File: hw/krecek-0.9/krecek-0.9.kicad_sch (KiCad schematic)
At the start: 3 parts, among them J1 USB_C_Receptacle_USB2.0, U1 RP2040, U2 W25Q128JVS

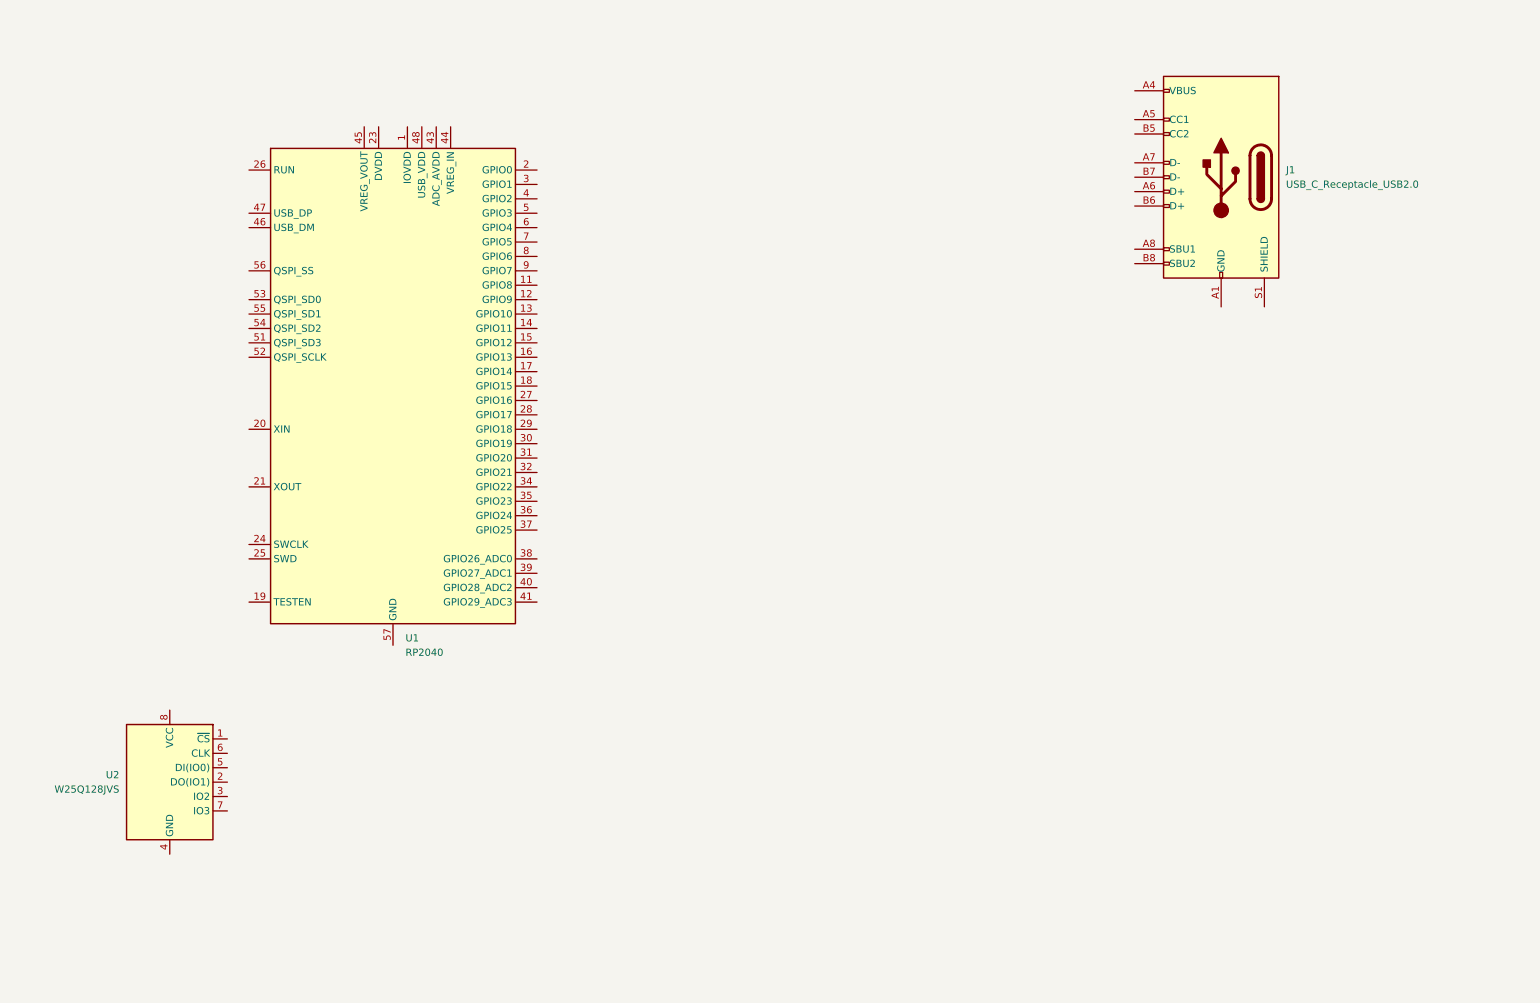
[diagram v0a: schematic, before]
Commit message: Expert hardware design *dab*
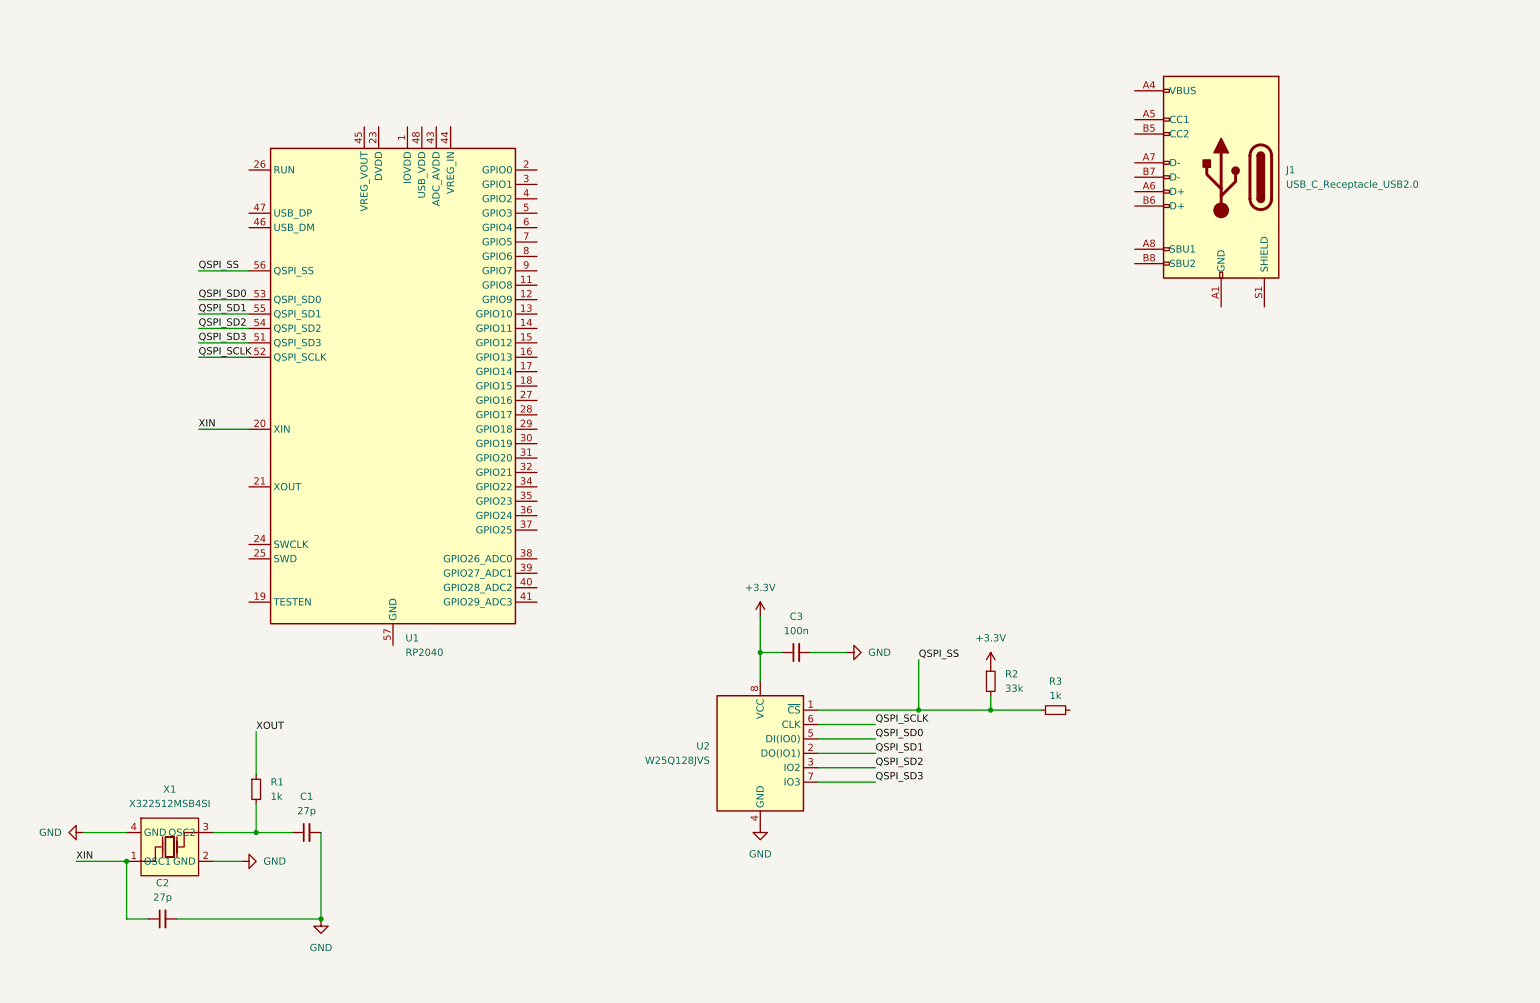
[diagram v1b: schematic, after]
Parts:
- added C1, C2: 27p, symbol Device:C_Small
- added C3: 100n, symbol Device:C_Small
- added R1, R3: 1k, symbol Device:R_Small
- added R2: 33k, symbol Device:R_Small
- added X1: X322512MSB4SI, LCSC:OSC-SMD_4P-L3.2-W2.5-BL, symbol LCSC:X322512MSB4SI
- J1: footprint (none) -> LCSC:USB-C-SMD_TYPEC-304J-BCP16; LCSC Part (none) -> C2835315
- U1: LCSC Part (none) -> C2040
- U2: LCSC Part (none) -> C97521
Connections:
- net XIN: now reaches U1.20 (XIN)
- net XIN: now also C2.1, X1.1 (OSC1)
- net QSPI_SD3: now reaches U1.51 (QSPI_SD3)
- net QSPI_SD3: now also U2.7 (IO3)
- net QSPI_SCLK: now reaches U1.52 (QSPI_SCLK)
- net QSPI_SCLK: now also U2.6 (CLK)
- net QSPI_SD0: now reaches U1.53 (QSPI_SD0)
- net QSPI_SD0: now also U2.5 (DI(IO0))
- net QSPI_SD2: now reaches U1.54 (QSPI_SD2)
- net QSPI_SD2: now also U2.3 (IO2)
- net QSPI_SD1: now reaches U1.55 (QSPI_SD1)
- net QSPI_SD1: now also U2.2 (DO(IO1))
- net QSPI_SS: now reaches U1.56 (QSPI_SS)
- net QSPI_SS: now also U2.1 (~{CS}), R2.2, R3.1
- net GND: now reaches U2.4 (GND)
- net GND: now also C1.2, C2.2, C3.2, X1.2 (GND), X1.4 (GND)
- net +3.3V: now reaches U2.8 (VCC)
- net +3.3V: now also C3.1, R2.1
- new net: C1.1, R1.2, X1.3 (OSC2)
- new net XOUT: R1.1
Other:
- moved on the sheet: U2

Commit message: expand design
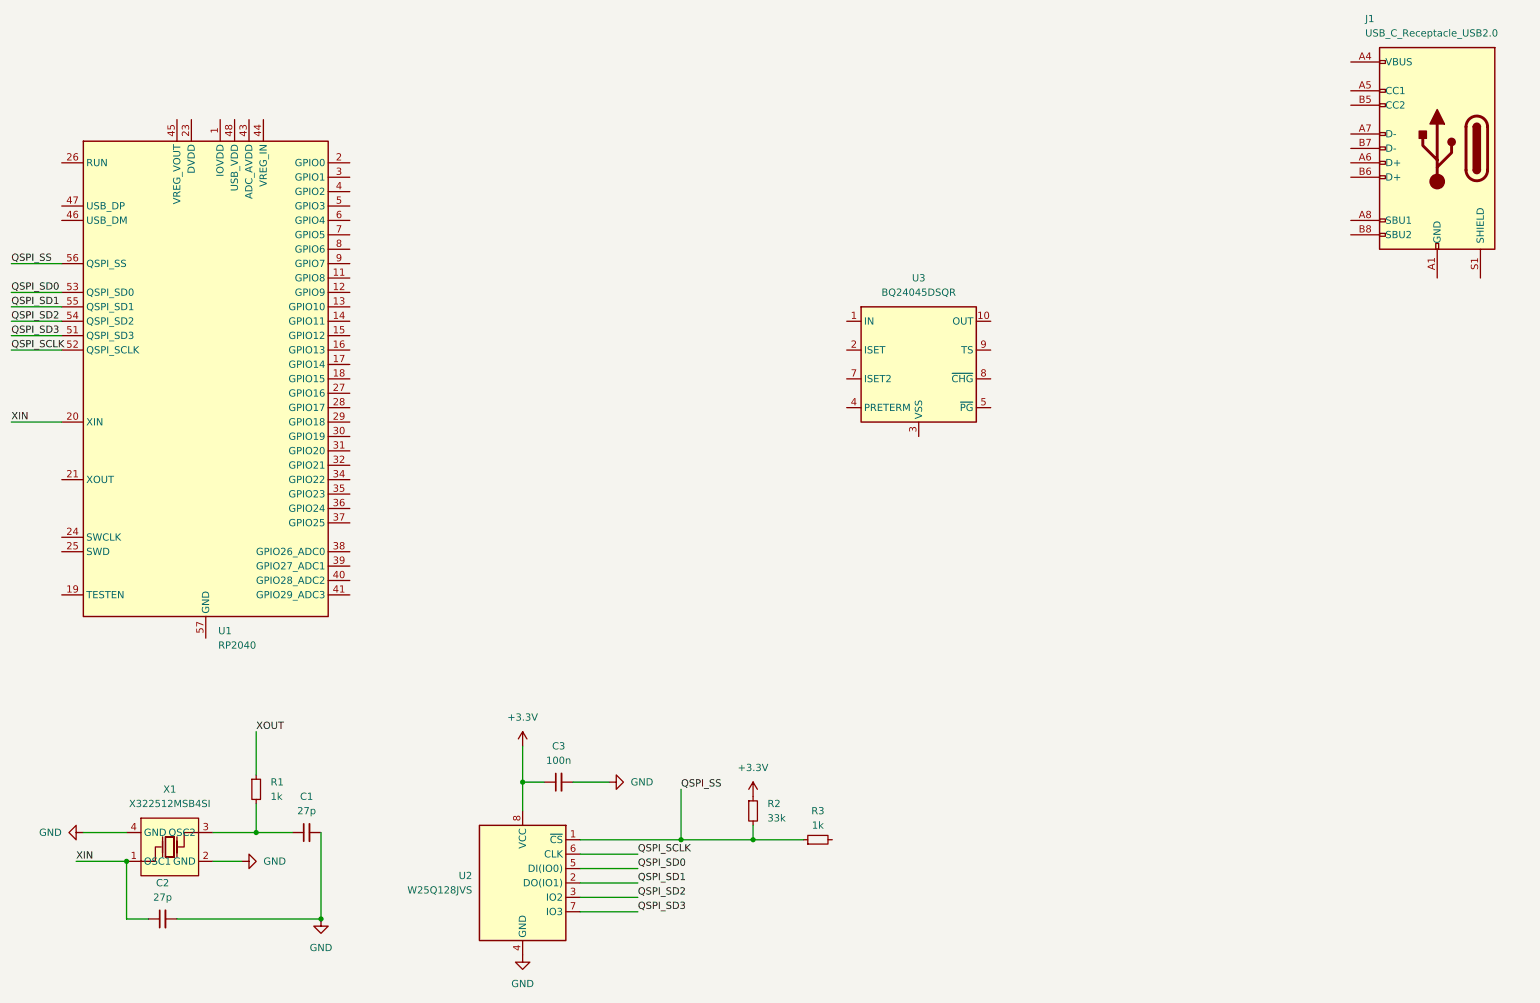
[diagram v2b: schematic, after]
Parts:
- added U3: BQ24045DSQR, LCSC:WSON-10_L2.0-W2.0-P0.40-BL-EP, symbol LCSC:BQ24045DSQR
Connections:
- new net: U3.11 (VSS), U3.3 (VSS)
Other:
- moved on the sheet: C3, J1, R2, R3, U1, U2

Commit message: assign GPIO pins
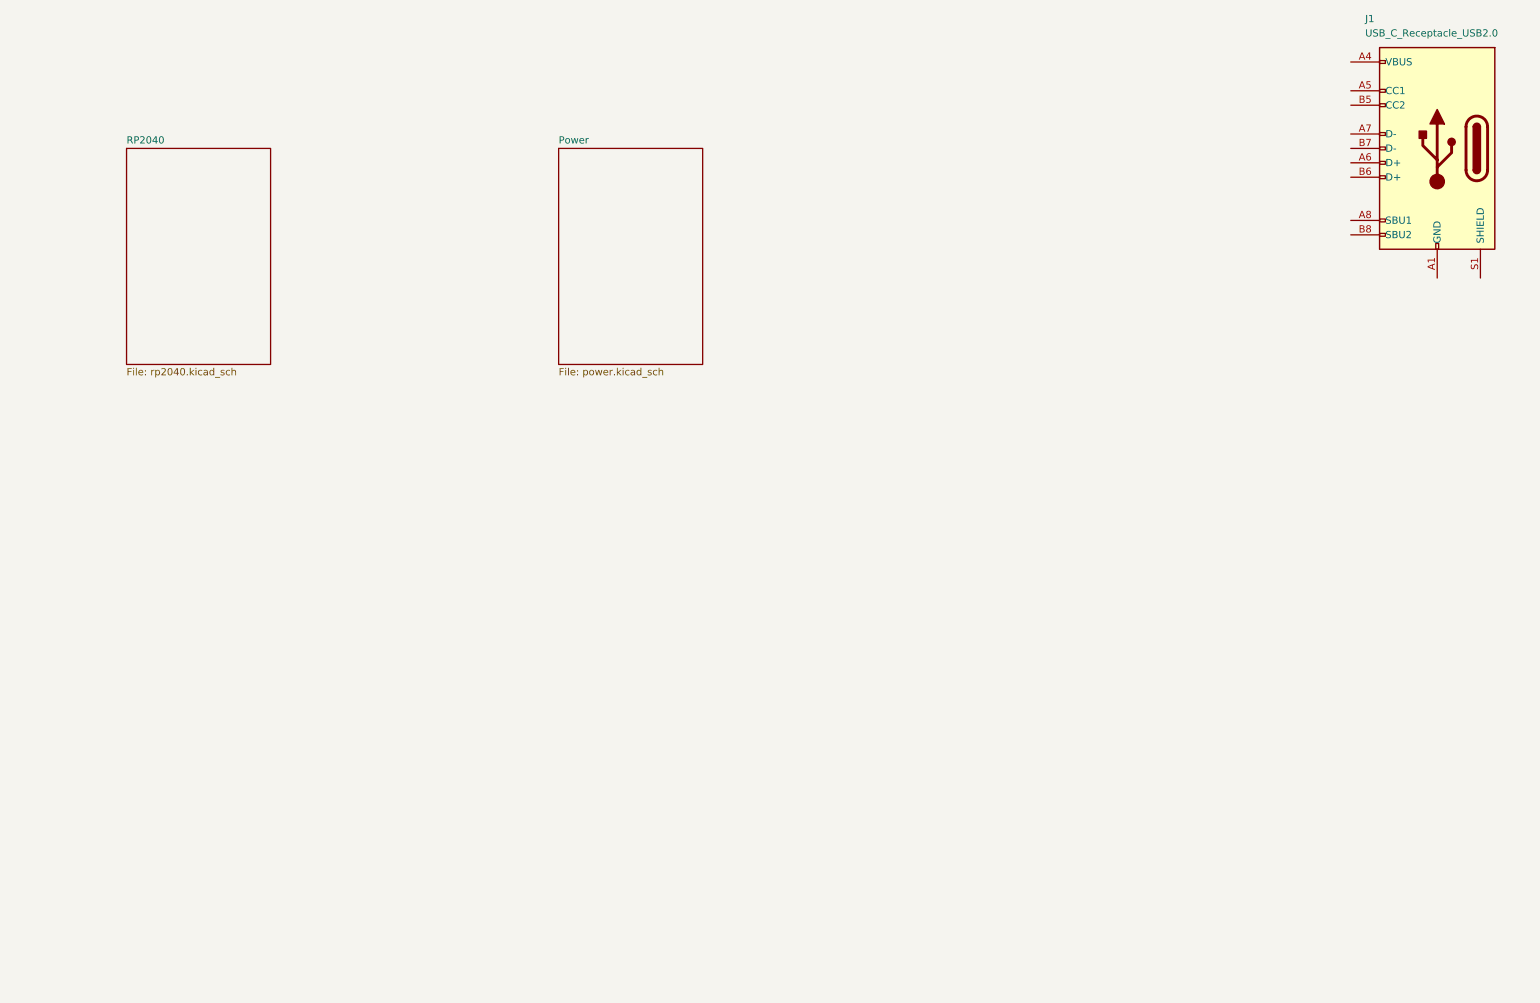
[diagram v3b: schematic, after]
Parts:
- removed C1, C2: 27p, symbol Device:C_Small
- removed C3: 100n, symbol Device:C_Small
- removed R1, R3: 1k, symbol Device:R_Small
- removed R2: 33k, symbol Device:R_Small
- removed U1: RP2040, Package_DFN_QFN:QFN-56-1EP_7x7mm_P0.4mm_EP3.2x3.2mm, symbol MCU_RaspberryPi:RP2040
- removed U2: W25Q128JVS, Package_SO:SOIC-8_5.23x5.23mm_P1.27mm, symbol Memory_Flash:W25Q128JVS
- removed U3: BQ24045DSQR, LCSC:WSON-10_L2.0-W2.0-P0.40-BL-EP, symbol LCSC:BQ24045DSQR
- removed X1: X322512MSB4SI, LCSC:OSC-SMD_4P-L3.2-W2.5-BL, symbol LCSC:X322512MSB4SI
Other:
- added sheet Power (power.kicad_sch)
- added sheet RP2040 (rp2040.kicad_sch)

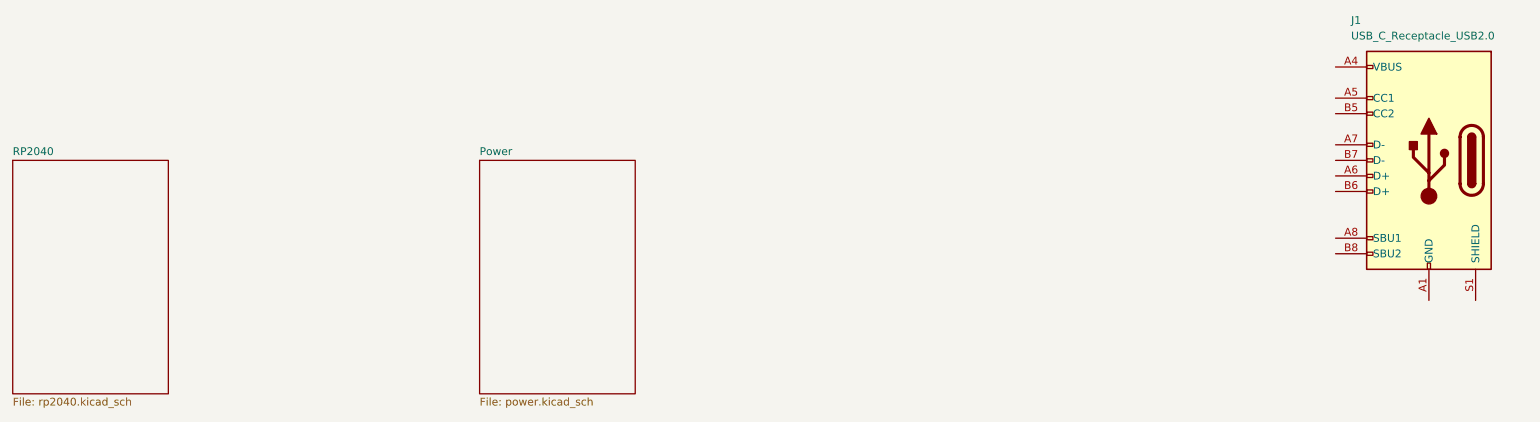
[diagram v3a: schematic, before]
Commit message: More work on power supply section
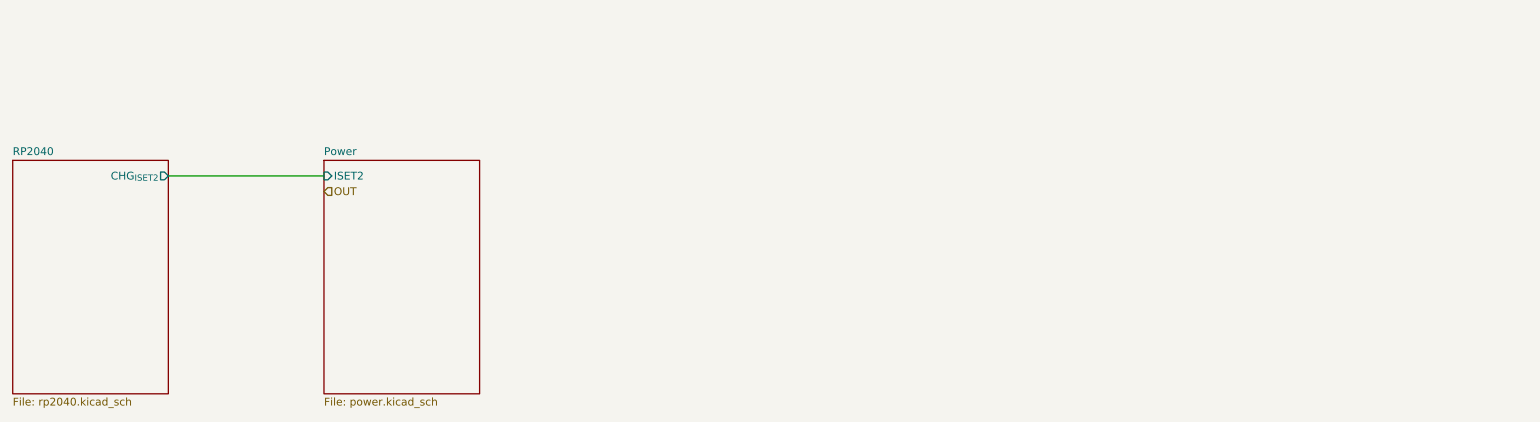
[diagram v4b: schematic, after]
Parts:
- removed J1: USB_C_Receptacle_USB2.0, LCSC:USB-C-SMD_TYPEC-304J-BCP16, symbol Connector:USB_C_Receptacle_USB2.0
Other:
- sheet Power ports: added ISET2; removed none
- sheet RP2040 ports: added CHG_{ISET2}; removed none
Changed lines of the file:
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@@
     (title "Křeček")
   )
-  (symbol (lib_id "Connector:USB_C_Receptacle_USB2.0") (at 269.24 38.1 0) (mirror y) (unit 1)
-    (in_bom yes) (on_board yes) (dnp no)
-    (property "Reference" "J1" (at 256.54 15.24 0)
-      (effects (font (size 1.27 1.27)) (justify right))
-    )
-    (property "Value" "USB_C_Receptacle_USB2.0" (at 256.54 17.78 0)
-      (effects (font (size 1.27 1.27)) (justify right))
-    )
-    (property "Footprint" "LCSC:USB-C-SMD_TYPEC-304J-BCP16" (at 265.43 38.1 0)
-      (effects (font (size 1.27 1.27)) hide)
-    )
-    (property "Datasheet" "https://www.usb.org/sites/default/files/documents/usb_type-c.zip" (at 265.43 38.1 0)
-      (effects (font (size 1.27 1.27)) hide)
-    )
-    (property "LCSC Part" "C2835315" (at 269.24 38.1 0)
-      (effects (font (size 1.27 1.27)) hide)
-    )
-    (pin "A1")
-    (pin "A12")
-    (pin "A4")
-    (pin "A5")
-    (pin "A6")
-    (pin "A7")
-    (pin "A8")
-    (pin "A9")
-    (pin "B1")
-    (pin "B12")
-    (pin "B4")
-    (pin "B5")
-    (pin "B6")
-    (pin "B7")
-    (pin "B8")
-    (pin "B9")
-    (pin "S1")
-    (instances
-      (project "krecek-0.9"
-        (path "/8888f37b-ecc2-47df-8824-4b4e1e726451"
-          (reference "J1") (unit 1)
-        )
-      )
-    )
+  (wire (pts (xy 63.5 40.64) (xy 88.9 40.64))
+    (stroke (width 0) (type default))
+  )
+  (hierarchical_label "OUT" (shape input) (at 88.9 43.18 0) (fields_autoplaced)
+    (effects (font (size 1.27 1.27)) (justify left))
   )
   (sheet (at 38.1 38.1) (size 25.4 38.1) (fields_autoplaced)
@@
       (effects (font (size 1.27 1.27)) (justify left top))
     )
+    (pin "CHG_{ISET2}" output (at 63.5 40.64 0)
+      (effects (font (size 1.27 1.27)) (justify right))
+    )
     (instances
       (project "krecek-0.9"
@@
     )
   )
-  (sheet (at 114.3 38.1) (size 25.4 38.1) (fields_autoplaced)
+  (sheet (at 88.9 38.1) (size 25.4 38.1) (fields_autoplaced)
     (stroke (width 0.1524) (type solid))
     (fill (color 0 0 0 0.0000))
-    (property "Sheetname" "Power" (at 114.3 37.3884 0)
+    (property "Sheetname" "Power" (at 88.9 37.3884 0)
       (effects (font (size 1.27 1.27)) (justify left bottom))
     )
-    (property "Sheetfile" "power.kicad_sch" (at 114.3 76.7846 0)
+    (property "Sheetfile" "power.kicad_sch" (at 88.9 76.7846 0)
       (effects (font (size 1.27 1.27)) (justify left top))
     )
+    (pin "ISET2" input (at 88.9 40.64 180)
+      (effects (font (size 1.27 1.27)) (justify left))
+    )
     (instances
